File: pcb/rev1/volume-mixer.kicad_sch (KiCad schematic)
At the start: 107 parts, among them CON1 TC2030-IDC, J1 Conn_01x10_Pin, J2 Conn_01x09_Pin, J3 Conn_01x09_Pin, J4 Conn_01x04_Pin, J5 Conn_01x04_Pin, J6 Conn_01x04_Pin, J7 Conn_01x04_Pin, J8 Conn_01x04_Pin, J9 Conn_01x04_Pin, Q1 2N7002, SW1 SW_Push, SW2 SW_Push, SW3 SW_Push, U1 STM32F302C8Tx, U2 24LC64, U3 XC6206PxxxMR, U4 XC6206PxxxMR, U5 PRTR5V0U2X, U6 TCA9548APWR, Y1 8MHz

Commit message: avancer du layout
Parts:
- removed C8, C9: 100nF, symbol Device:C_Small
- removed D2, D5, D6, D8: LED, symbol Device:LED
- removed J2, J3: Conn_01x09_Pin, symbol Connector:Conn_01x09_Pin
- removed Q1: 2N7002, Package_TO_SOT_SMD:SOT-23, symbol Transistor_FET:2N7002
- removed R16, R17, R19, R20, R22: 1k2, symbol Device:R_Small
- added D10, D11, D12, D13: LED, A_Please:LED C516299, symbol Device:LED
- added J3: Conn_01x10_Pin, Connector_PinHeader_1.27mm:PinHeader_2x05_P1.27mm_Vertical, symbol Connector:Conn_01x10_Pin
- added J4: Conn_01x04_Pin, Connector_PinHeader_2.54mm:PinHeader_1x04_P2.54mm_Vertical, symbol Connector:Conn_01x04_Pin
- added J5: JST, A_random_part:JST-SR-4, symbol Connector:Conn_01x04_Socket
- added Q1, Q10, Q3, Q7, Q8, Q9: NMOS, Package_TO_SOT_SMD:SOT-23, symbol Simulation_SPICE:NMOS
- added R15, R61, R64, R65, R67, R68, R70, R71, R73, R74: 100, Resistor_SMD:R_0603_1608Metric, symbol Device:R_Small
- added R62, R63, R66, R69, R72: 10K, Resistor_SMD:R_0603_1608Metric, symbol Device:R_Small
- C1, C2, C3, C4, C5, C6, C7: footprint Capacitor_SMD:C_0402_1005Metric -> Capacitor_SMD:C_0603_1608Metric
- C10: renamed from C12; footprint (none) -> Capacitor_SMD:C_0603_1608Metric
- C11: renamed from C13; footprint (none) -> Capacitor_SMD:C_0603_1608Metric
- C12: renamed from C14; footprint (none) -> Capacitor_SMD:C_0603_1608Metric
- C13: renamed from C15; value C_Small -> 100nF; footprint (none) -> Capacitor_SMD:C_0603_1608Metric
- C14: renamed from C16; footprint Capacitor_SMD:C_0402_1005Metric -> Capacitor_SMD:C_0603_1608Metric
- C15: renamed from C17; footprint (none) -> Capacitor_SMD:C_0603_1608Metric
- C16: renamed from C18; footprint Capacitor_SMD:C_0402_1005Metric -> Capacitor_SMD:C_0603_1608Metric
- C17: renamed from C19; footprint Capacitor_SMD:C_0402_1005Metric -> Capacitor_SMD:C_0603_1608Metric
- C18: renamed from C20; footprint Capacitor_SMD:C_0402_1005Metric -> Capacitor_SMD:C_0603_1608Metric
- C19: renamed from C21; footprint Capacitor_SMD:C_0402_1005Metric -> Capacitor_SMD:C_0603_1608Metric
- C20: renamed from C22; footprint Capacitor_SMD:C_0402_1005Metric -> Capacitor_SMD:C_0603_1608Metric
- C21: renamed from C23; footprint (none) -> Capacitor_SMD:C_0603_1608Metric
- C22: renamed from C24; footprint (none) -> Capacitor_SMD:C_0603_1608Metric
- C23: renamed from C25; footprint (none) -> Capacitor_SMD:C_0603_1608Metric
- C24: renamed from C26; footprint (none) -> Capacitor_SMD:C_0603_1608Metric
- C25: renamed from C27; footprint (none) -> Capacitor_SMD:C_0603_1608Metric
- C26: renamed from C28; footprint (none) -> Capacitor_SMD:C_0603_1608Metric
- C27: renamed from C29; footprint (none) -> Capacitor_SMD:C_0603_1608Metric
- C28: renamed from C30; footprint (none) -> Capacitor_SMD:C_0603_1608Metric
- C29: renamed from C31; footprint (none) -> Capacitor_SMD:C_0603_1608Metric
- C30: renamed from C32; footprint (none) -> Capacitor_SMD:C_0603_1608Metric
- C8: renamed from C11; footprint Capacitor_SMD:C_0402_1005Metric -> Capacitor_SMD:C_0603_1608Metric
- C9: renamed from C10; value C_Small -> 100nF; footprint (none) -> Capacitor_SMD:C_0603_1608Metric
- D1: renamed from D9; footprint (none) -> A_Please:LED C516299
- D3: footprint (none) -> A_Please:LED C516299
- J1: renamed from J4; footprint (none) -> Connector_PinHeader_2.54mm:PinHeader_1x04_P2.54mm_Vertical
- J10: renamed from J9; footprint (none) -> A_Please:Screen 0.91 I2C
- J2: renamed from J1; footprint (none) -> Connector_PinHeader_2.54mm:PinHeader_1x10_P2.54mm_Vertical
- J6: renamed from J5; footprint (none) -> A_Please:Screen 0.91 I2C
- J7: renamed from J6; footprint (none) -> A_Please:Screen 0.91 I2C
- J8: renamed from J7; footprint (none) -> A_Please:Screen 0.91 I2C
- J9: renamed from J8; footprint (none) -> A_Please:Screen 0.91 I2C
- R1, R2: value R_Small -> 10k; footprint (none) -> Resistor_SMD:R_0603_1608Metric
- R10, R24, R25, R26, R27, R28, R29, R30, R31, R32, R33, R34, R35, R36, R37, R38, R39, R6, R7, R8, R9: footprint (none) -> Resistor_SMD:R_0603_1608Metric
- R11, R12, R3, R4, R5: footprint Resistor_SMD:R_0402_1005Metric -> Resistor_SMD:R_0603_1608Metric
- R13: renamed from R23; footprint (none) -> Resistor_SMD:R_0603_1608Metric
- R16: renamed from R15; footprint (none) -> Resistor_SMD:R_0603_1608Metric
- R17: renamed from R13; footprint (none) -> Resistor_SMD:R_0603_1608Metric
- R18: renamed from R14; footprint (none) -> Resistor_SMD:R_0603_1608Metric
- R19: renamed from R18; footprint (none) -> Resistor_SMD:R_0603_1608Metric
- R22: renamed from R21; footprint (none) -> Resistor_SMD:R_0603_1608Metric
- SW1, SW3: footprint (none) -> Button_Switch_SMD:SW_SPST_SKQG_WithStem
- TP1, TP2, TP3, TP4, TP5: footprint (none) -> TestPoint:TestPoint_Keystone_5015_Micro_Mini
- U2: footprint (none) -> Package_SO:SOIC-8_3.9x4.9mm_P1.27mm
- renumbered D1 to D4, D4 to D5, D7 to D8
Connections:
- net +3V3: now also J3.1 (Pin_1), J4.1 (Pin_1)
- net D+: now also J5.3 (Pin_3)
- net D-: now also J5.2 (Pin_2)
- net GND: now also J3.3 (Pin_3), J3.5 (Pin_5), J3.9 (Pin_9), J4.4 (Pin_4), J5.4 (Pin_4), Q1.3 (S), Q10.3 (S), Q3.3 (S), Q7.3 (S), Q8.3 (S), Q9.3 (S), R62.1, R63.1, R66.1, R69.1, R72.1; no longer D3.1 (K)
- net Mute0Led: now also R61.1, R62.2
- net Mute1Led: now also R63.2, R64.1
- net Mute2Led: now also R66.2, R67.1
- net Mute3Led: now also R69.2, R70.1
- net Mute4Led: now also R72.2, R73.1
- net RESET: now also J3.10 (Pin_10), Q1.1 (D)
- net SCL: now also J4.2 (Pin_2)
- net SDA: now also J4.3 (Pin_3)
- net SWCLK: now also J3.4 (Pin_4)
- net SWDIO: now also J3.2 (Pin_2)
- net VBUS: now also J5.1 (Pin_1), R15.1, R65.1, R68.1, R71.1, R74.1
- net at C14.2, R5.1: now also Q1.2 (G)
- net at D3.2 (A): now also R15.2
- new net: D11.2 (A), R68.2
- new net: D13.1 (K), Q10.1 (D)
- new net: D13.2 (A), R74.2
- new net: D10.2 (A), R65.2
- new net: D11.1 (K), Q8.1 (D)
- new net: Q8.2 (G), R67.2
- new net: Q10.2 (G), R73.2
- new net: D10.1 (K), Q7.1 (D)
- new net: Q7.2 (G), R64.2
- new net: Q9.2 (G), R70.2
- new net: D12.1 (K), Q9.1 (D)
- new net: D12.2 (A), R71.2
- new net: D3.1 (K), Q3.1 (D)
- new net: Q3.2 (G), R61.2
- no-connect marks 2 -> 3
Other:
- note removed: "3V3 Decoupling"
- moved on the sheet: C1, C10, C12, C13, C14, C15, C16, C17, C18, C19, C2, C20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

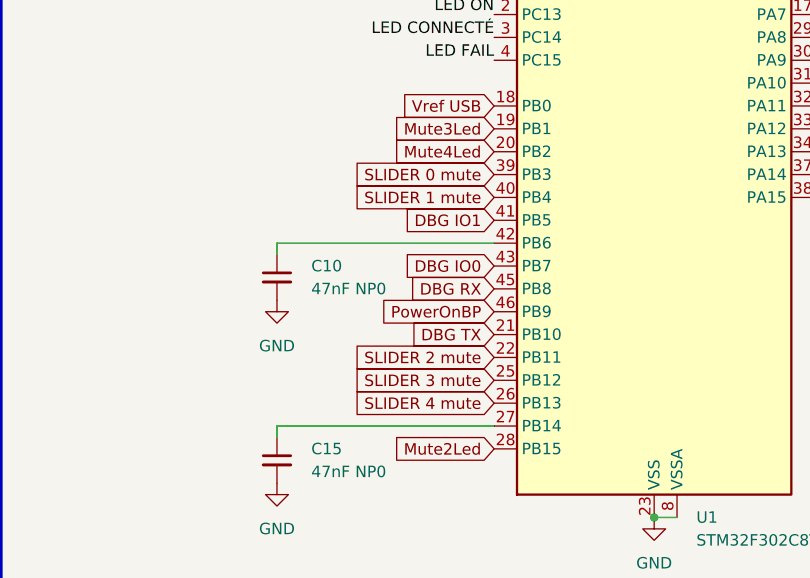
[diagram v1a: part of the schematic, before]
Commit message: blabla
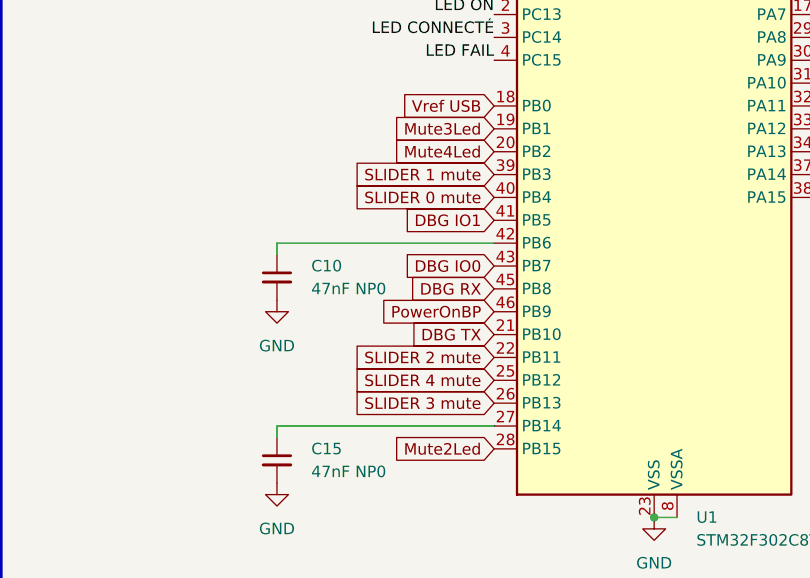
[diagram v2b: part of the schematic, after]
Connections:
- net SLIDER 0 mute : now also U1.40 (PB4); no longer U1.39 (PB3)
- net SLIDER 1 mute : now also U1.39 (PB3); no longer U1.40 (PB4)
- net SLIDER 3 mute : now also U1.26 (PB13); no longer U1.25 (PB12)
- net SLIDER 4 mute : now also U1.25 (PB12); no longer U1.26 (PB13)
